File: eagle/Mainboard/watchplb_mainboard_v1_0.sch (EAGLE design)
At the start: 214 parts, among them IC2 BM70BLES1FC2-0B03AA, IC3 LM1117DTX-ADJ-12V, IC5 LM1117DTX-ADJ-10V, IC6 LM1117DTX-ADJ-3V3, J3 BNCPTH, Q1 8MHz / LFXTAL020423Reel, Q2 BC817-25SMD, Q3 DMN3023L-7, Q4 16MHz_LFXTAL051370Reel, Q5 CSD18534Q5A, Q6 CSD18534Q5A, Q7 DMN3023L-7, U1 MCP111-XXXXX/TO, U2 STM32L073RZ, U3 MCP2200-I/SS, U4 TPD3E001DRLR, U5 BQ7790504

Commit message: Änderungen laut Besprechung mit Armin (soweit ich mich erinnern kann, ist schon ne woche her)
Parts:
- removed U$1: AX5031, Hick:AX5031
- removed U$3: LT1513, Hick:LT1513
- added IC1: LT1513, Hick:LT1513
- added IC4: AX5031, Hick:AX5031
- BAT_PACK_POS: value PTR1B2,54 -> PTR1B1,27; device testpad:PTR1B2,54 -> testpad:PTR1B1,27
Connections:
- net ANT_N: now also IC4.ANTN; no longer U$1.ANTN
- net ANT_P: now also IC4.ANTP; no longer U$1.ANTP
- net CHARGER_SS: now also IC1.S/S; no longer U$3.S/S
- net GND: now also IC1.GND, IC4.GND_PAD; no longer U$1.GND_PAD, U$3.GND
- net INT_POWER: now also IC4.VDD1, IC4.VDD2, IC4.VREG; no longer U$1.VDD1, U$1.VDD2, U$1.VREG
- net N$33: now also IC4.CLOCK16P; no longer U$1.CLOCK16P
- net N$34: now also IC4.CLOCK16N; no longer U$1.CLOCK16N
- net N$37: now also IC4.SYSCLK; no longer U$1.SYSCLK
- net N$61: now also IC1.VSW; no longer U$3.VSW
- net N$69: now also IC1.VIN; no longer U$3.VIN
- net N$72: now also IC1.VC; no longer U$3.VC
- net N$76: now also IC1.IFB; no longer U$3.IFB
- net N$77: now also IC1.VFB; no longer U$3.VFB
- net N$82: now also IC4.VDD_IO; no longer U$1.VDD_IO
- net SPI2_CLK: now also IC4.CLK; no longer U$1.CLK
- net SPI2_IRQ: now also IC4.IRQ; no longer U$1.IRQ
- net SPI2_MISO: now also IC4.MISO_SDO; no longer U$1.MISO_SDO
- net SPI2_MOSI: now also IC4.MOSI_SDI; no longer U$1.MOSI_SDI
- net SPI2_SEL_RFTX: now also IC4.SEL; no longer U$1.SEL
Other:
- note added: "Battery Protection"
- note added: "Linear Voltage Regulators"

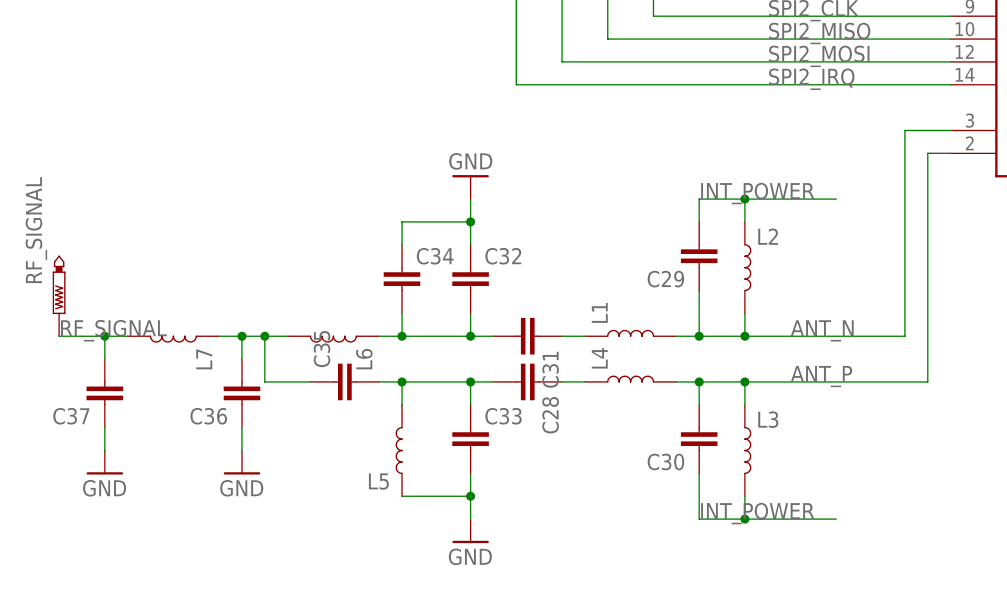
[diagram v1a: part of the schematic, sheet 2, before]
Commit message: started BOM
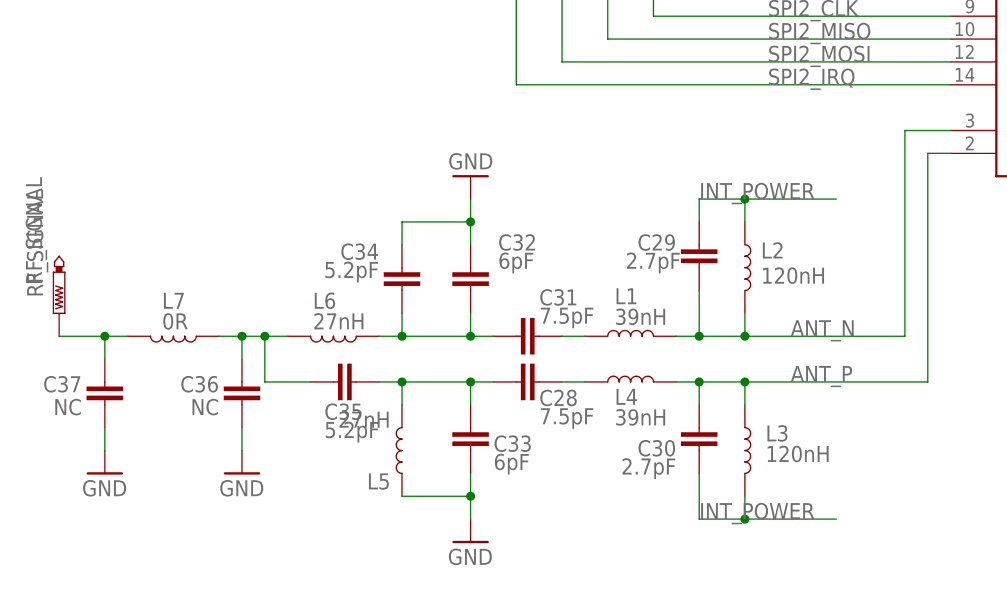
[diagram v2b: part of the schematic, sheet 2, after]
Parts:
- C28, C31: value (none) -> 7.5pF
- C29, C30: value (none) -> 2.7pF
- C32, C33: value (none) -> 6pF
- C34, C35: value (none) -> 5.2pF
- C36, C37: value (none) -> NC
- L1, L4: value INDUCTOR-0805-3.3UH -> 39nH
- L2, L3: value INDUCTOR-0805-3.3UH -> 120nH
- L5, L6: value INDUCTOR-0805-3.3UH -> 27nH
- L7: value INDUCTOR-0805-3.3UH -> 0R
